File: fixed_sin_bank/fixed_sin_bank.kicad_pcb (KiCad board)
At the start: 2 copper layers, 18.8 x 116.8 mm, 101 parts, among them J101 Conn_02x05_Odd_Even, J201 AudioJack2_SwitchT, J301 AudioJack2_SwitchT, J401 AudioJack2_SwitchT, J501 AudioJack2_SwitchT, J601 AudioJack2_SwitchT, J701 AudioJack2_SwitchT, U201 TL071HDBV, U301 TL071HDBV, U401 TL071HDBV, U501 TL071HDBV, U601 TL071HDBV, U701 TL071HDBV

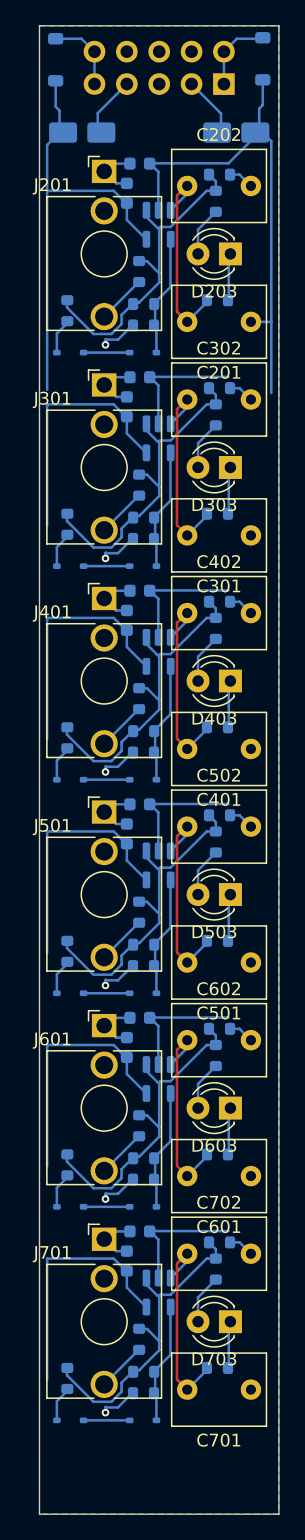
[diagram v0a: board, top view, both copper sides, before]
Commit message: First draft of pcb
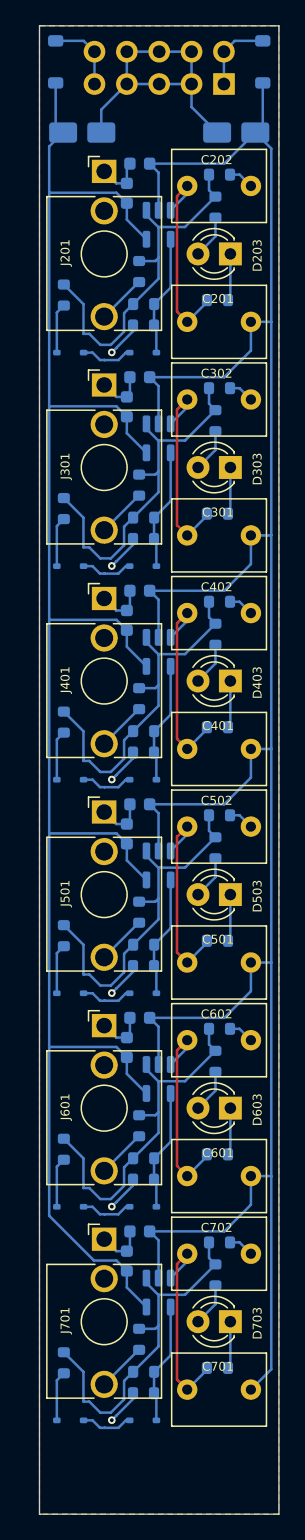
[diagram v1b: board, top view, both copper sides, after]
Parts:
- moved R505 1.26 mm to (134.5, 104.2)
- moved R305 1.26 mm to (134.5, 70.7)
- moved R405 1.26 mm to (134.5, 87.4)
- moved R605 1.26 mm to (134.5, 121.0)
- moved R705 1.26 mm to (134.5, 137.7)
- moved R205 1.26 mm to (134.5, 53.9)
- moved R407 0.46 mm to (146.4, 80.5)
- moved R507 0.46 mm to (146.4, 97.3)
- moved R307 0.46 mm to (146.4, 63.8)
- moved R607 0.46 mm to (146.4, 114.1)
- moved R707 0.46 mm to (146.4, 130.8)
- moved R207 0.46 mm to (146.4, 47.0)
- moved D102 0.24 mm to (150.1, 35.6)
- moved D101 0.17 mm to (133.9, 35.6)
- turned C101 to 0 degrees
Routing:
- net VEE: track 91.0 -> 200.4 mm
- net VCC: track 133.0 -> 150.6 mm
- net GND: track 77.5 -> 86.5 mm
- net Net-(R203-Pad2): track 26.4 -> 28.6 mm
- net Net-(R303-Pad2): track 26.4 -> 28.6 mm
- net Net-(R603-Pad2): track 26.4 -> 28.6 mm
- net Net-(R403-Pad2): track 26.4 -> 28.6 mm
- net Net-(R503-Pad2): track 26.4 -> 28.6 mm
- net Net-(R703-Pad2): track 26.4 -> 28.6 mm
- net Net-(D702-K): track 2.62 -> 3.92 mm
- net Net-(D502-K): track 2.62 -> 3.92 mm
- net Net-(D302-K): track 2.62 -> 3.92 mm
- net Net-(D202-K): track 2.62 -> 3.92 mm
- net Net-(D402-K): track 2.62 -> 3.92 mm
- net Net-(D602-K): track 2.62 -> 3.92 mm
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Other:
- board text added: "fixed sin bank v1.0 www.birchavenue.org"
